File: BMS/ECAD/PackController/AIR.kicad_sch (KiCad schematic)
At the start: 33 parts, among them J1 Conn_01x08, K401 AIR_P, K402 AIR_N, Q3 BC846, Q4 BC846, Q402 DMP4065S-7, Q404 DMP4065S-7, U401 ADCMP393ARUZ

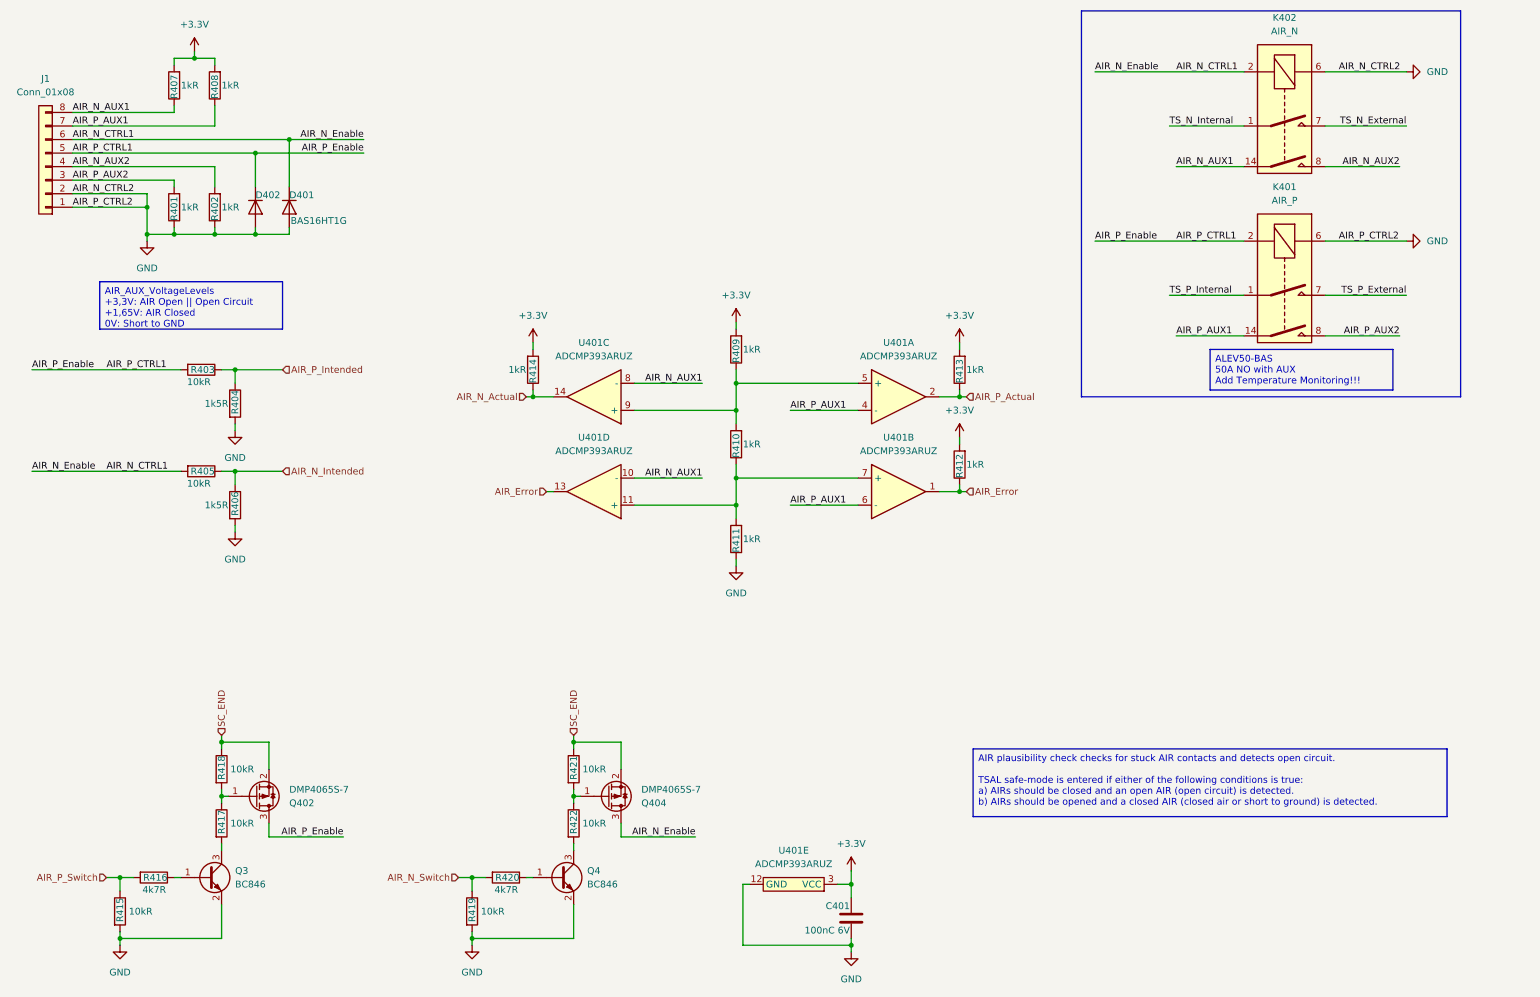
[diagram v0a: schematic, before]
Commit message: schematic finished, review tbd
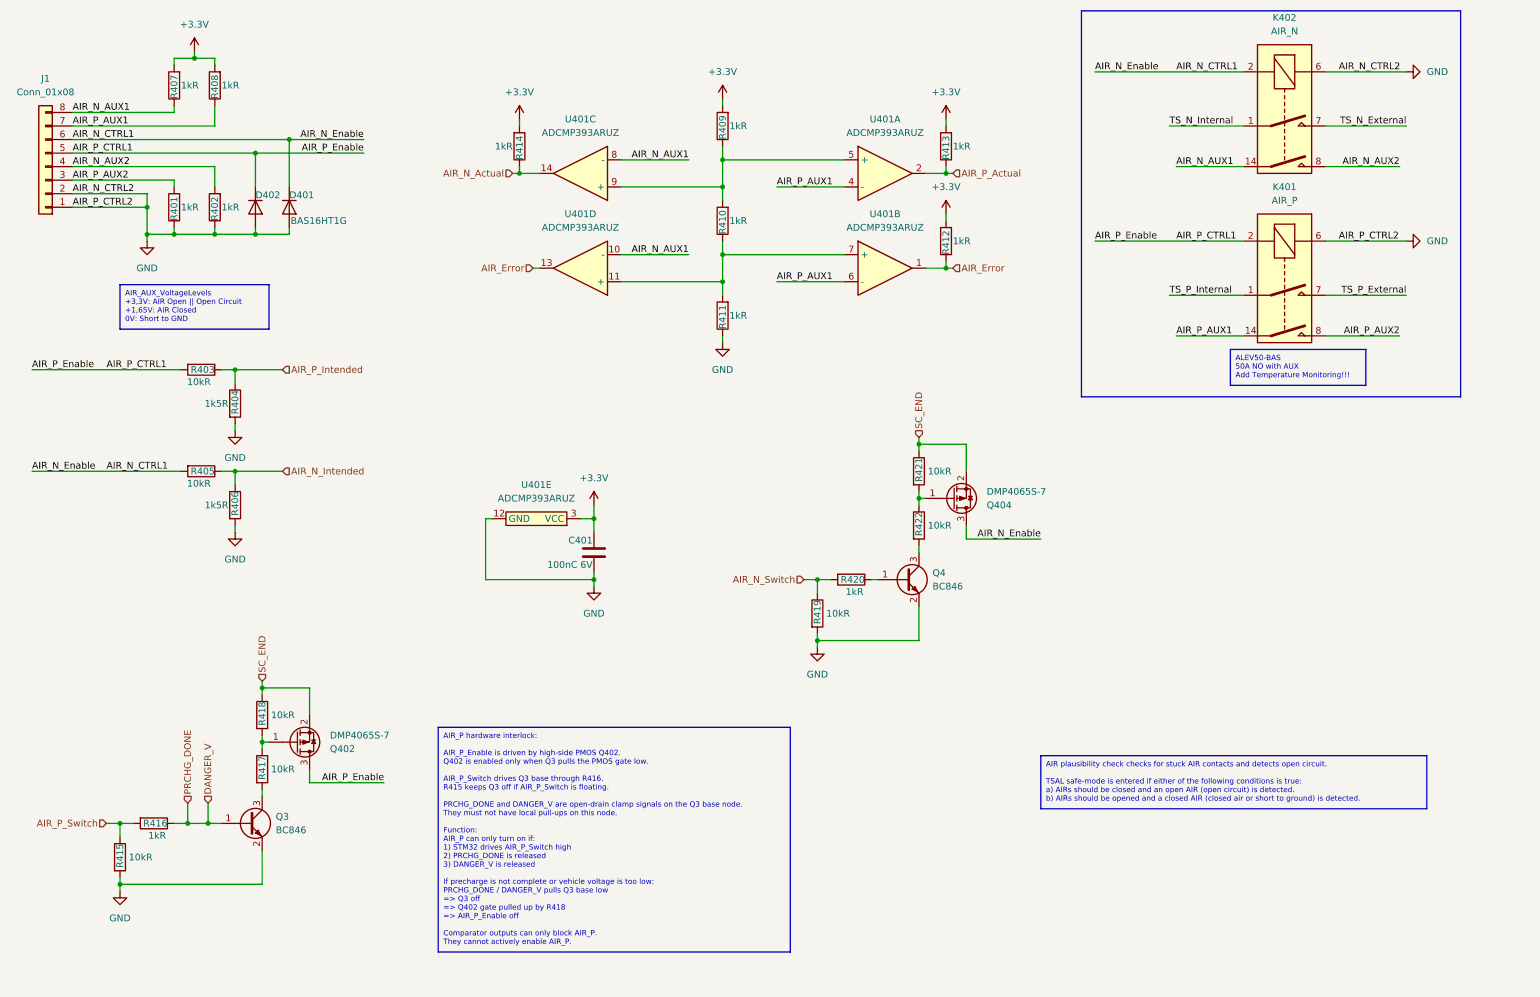
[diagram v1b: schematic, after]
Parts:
- R416, R420: value 4k7R -> 1kR
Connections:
- net DANGER_V: now reaches Q3.1 (B), R416.1
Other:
- moved on the sheet: C401, Q3, Q4, Q402, Q404, R409, R410, R411, R412, R413, R414, R415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
